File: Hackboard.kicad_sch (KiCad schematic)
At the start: 66 parts, among them J1 Conn_01x31_Socket, J2 Micro_SD_Card, J3 Conn_01x31_Socket, J5 Conn_02x02_Counter_Clockwise, J6 USB_C_Receptacle_USB2.0_16P, J7 Barrel_Jack_Switch, Q1 NMOS, Q2 NMOS, Q3 NMOS, SW1 SW_DPST, U1 NCP164CSN330T1G, U2 AP63205WU, U3 STM32L476RGT6, U4 74LVC4245APW, U5 74LVC4245APW, U6 74LVC4245APW, U7 USBLC6-2SC6, U8 74LVC4245APW, U9 74LVC4245APW

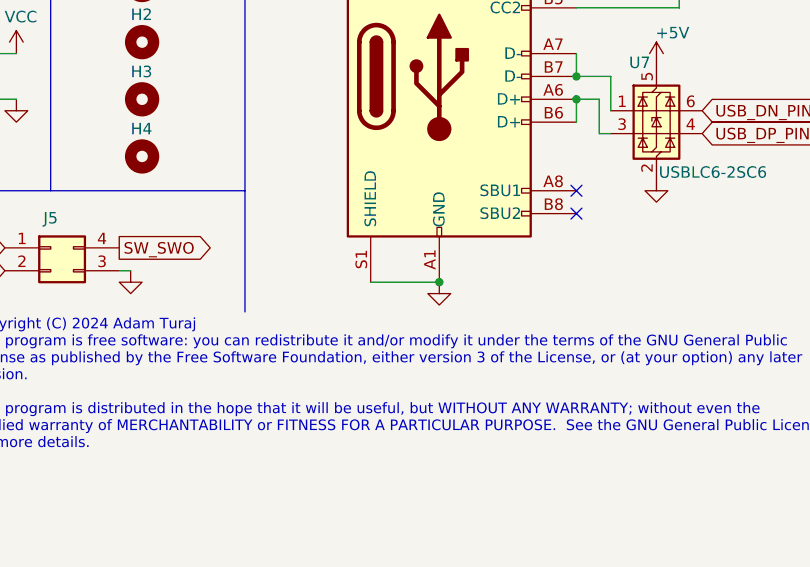
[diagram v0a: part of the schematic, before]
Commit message: Route power
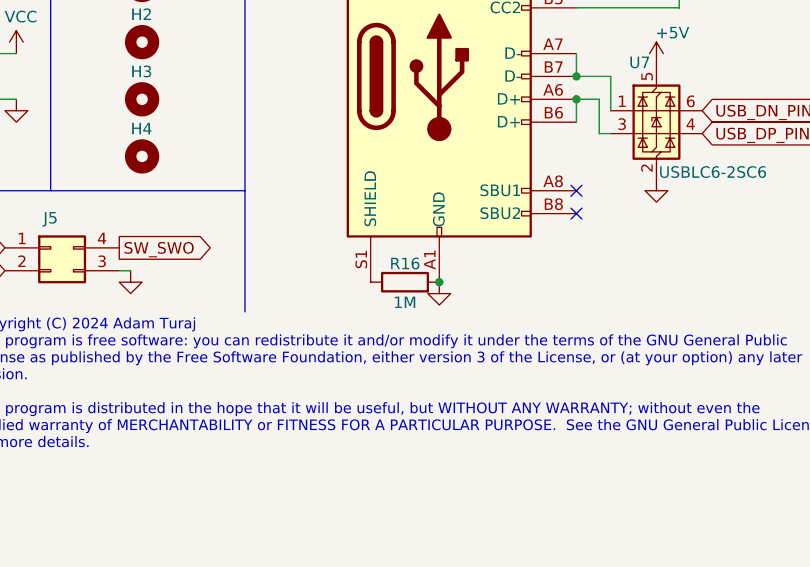
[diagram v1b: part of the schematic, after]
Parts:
- added R16: 1M, symbol Device:R
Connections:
- net GND: now also R16.2; no longer J6.S1 (SHIELD)
- new net: J6.S1 (SHIELD), R16.1
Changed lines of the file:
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@@
 	)
 	(junction
+		(at 229.87 162.56)
+		(diameter 0)
+		(color 0 0 0 0)
+	)
+	(junction
 		(at 246.38 106.68)
 		(diameter 0)
@@
 	)
 	(junction
-		(at 229.87 162.56)
-		(diameter 0)
-		(color 0 0 0 0)
-	)
-	(junction
 		(at 62.23 19.05)
 		(diameter 0)
@@
 		)
 	)
-	(wire
-		(pts
-			(xy 222.25 162.56) (xy 229.87 162.56)
-		)
-		(stroke
-			(width 0)
-			(type default)
-		)
-	)
 	(polyline
 		(pts
@@
 					(unit 1)
 				)
+			)
+		)
+	)
+	(symbol
+		(lib_id "Device:R")
+		(at 226.06 162.56 90)
+		(unit 1)
+		(exclude_from_sim no)
+		(in_bom yes)
+		(on_board yes)
+		(dnp no)
+		(property "Reference" "R16"
+			(at 226.06 160.528 90)
+			(effects
+				(font
+					(size 1.27 1.27)
+				)
+			)
+		)
+		(property "Value" "1M"
+			(at 226.06 164.846 90)
+			(effects
+				(font
+					(size 1.27 1.27)
+				)
+			)
+		)
+		(property "Footprint" ""
+			(at 226.06 164.338 90)
+			(effects
+				(font
+					(size 1.27 1.27)
+				)
+				(hide yes)
+			)
+		)
+		(property "Datasheet" "~"
+			(at 226.06 162.56 0)
+			(effects
+				(font
+					(size 1.27 1.27)
+				)
+				(hide yes)
+			)
+		)
+		(property "Description" "Resistor"
+			(at 226.06 162.56 0)
+			(effects
+				(font
+					(size 1.27 1.27)
+				)
+				(hide yes)
+			)
+		)
+		(pin "2"
+		)
+		(pin "1"
+		)
+		(instances
+			(project "Hackboard"
+				(path "/478098fb-f4b2-4694-bef3-d53baad1e8cf"
+					(reference "R16")
+					(unit 1)
+				)
